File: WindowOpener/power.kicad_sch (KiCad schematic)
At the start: 39 parts, among them J10 Motor1, J11 Batt_Conn, J12 Batt_Conn, J13 Batt_Conn, J14 Motor2, J3 Batt_Conn, J4 Batt_Conn, J5 Batt_Conn, J6 Batt_Conn, J7 Batt_Conn, J8 Batt_Conn, J9 Batt_Conn, U3 AZ1117CH2-3.3, U4 MIC2288YD5-TR, U5 DRV8220DRL, U6 DRV8220DRL, U7 MIC2288YD5-TR

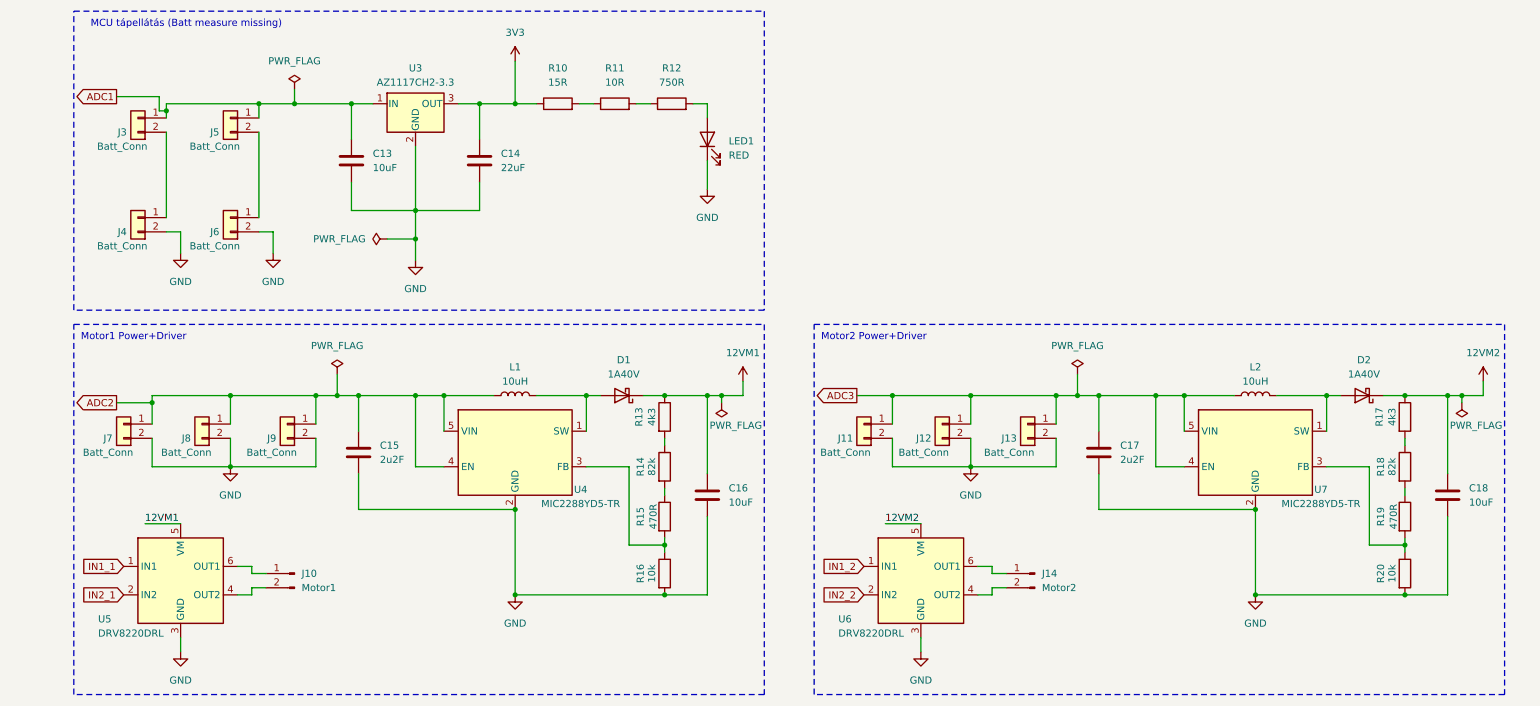
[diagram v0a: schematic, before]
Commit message: v0.5
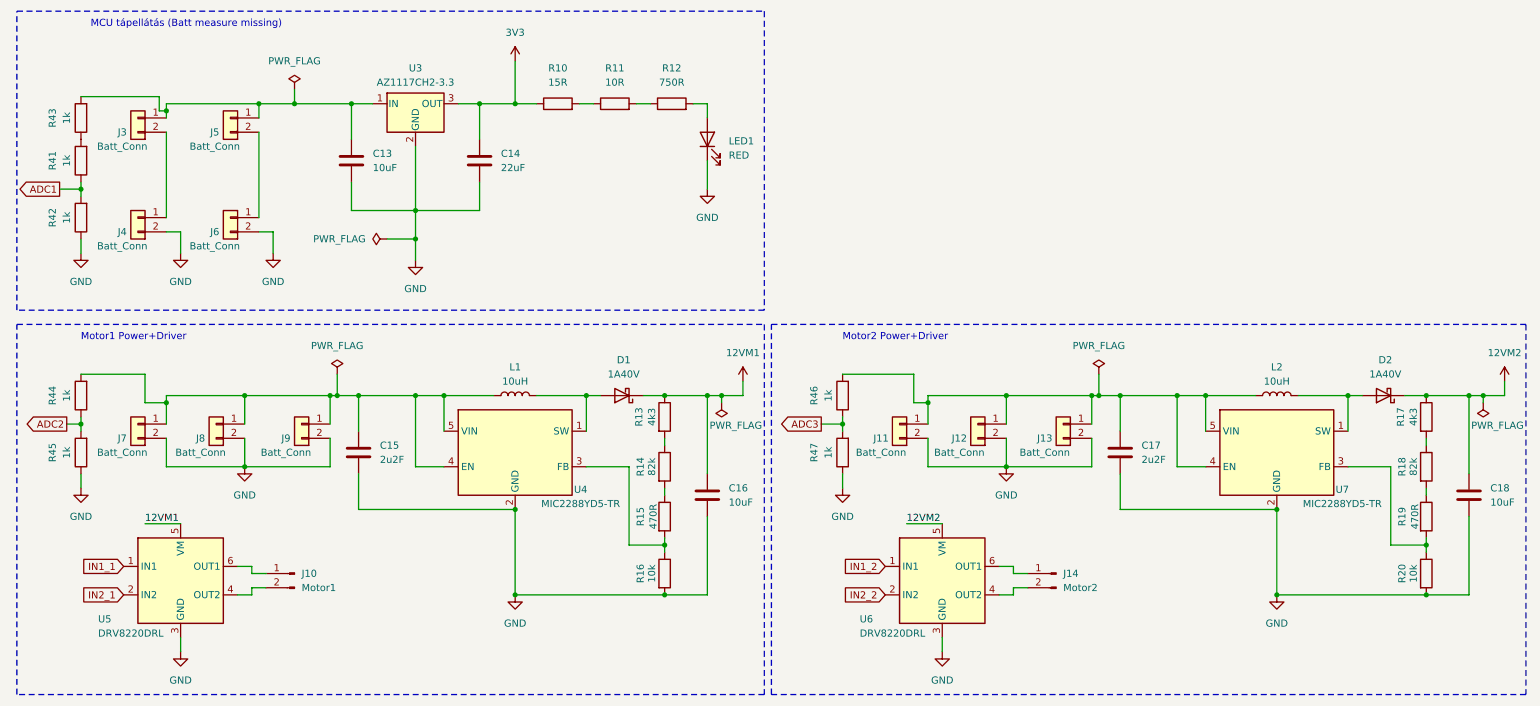
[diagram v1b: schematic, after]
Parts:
- added R41, R42, R43, R44, R45, R46, R47: 1k, Resistor_SMD:R_2010_5025Metric_Pad1.40x2.65mm_HandSolder, symbol Device:R
- U5, U6: Store link (none) -> https://www.ti.com/product/DRV8220?login-check=true#order-q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
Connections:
- net ADC1: now also R41.1, R42.2; no longer C13.1, J3.1 (Pin_2), J5.1 (Pin_2), U3.1 (IN)
- net ADC2: now also R44.1, R45.2; no longer C15.1, J7.1 (Pin_2), J8.1 (Pin_2), J9.1 (Pin_2), L1.1, U4.4 (EN), U4.5 (VIN)
- net ADC3: now also R46.1, R47.2; no longer C17.1, J11.1 (Pin_2), J12.1 (Pin_2), J13.1 (Pin_2), L2.1, U7.4 (EN), U7.5 (VIN)
- net GND: now also R42.1, R45.1, R47.1
- new net: C13.1, J3.1 (Pin_2), J5.1 (Pin_2), R43.2, U3.1 (IN)
- new net: C17.1, J11.1 (Pin_2), J12.1 (Pin_2), J13.1 (Pin_2), L2.1, R46.2, U7.4 (EN), U7.5 (VIN)
- new net: R41.2, R43.1
- new net: C15.1, J7.1 (Pin_2), J8.1 (Pin_2), J9.1 (Pin_2), L1.1, R44.2, U4.4 (EN), U4.5 (VIN)
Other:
- moved on the sheet: C17, C18, D2, J11, J12, J13, J14, J7, J8, J9, L2, R17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
